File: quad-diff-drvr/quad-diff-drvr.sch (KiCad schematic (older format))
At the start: 53 parts, among them J1 Raspberry_Pi_2_3, J2 Conn_01x04, J3 Conn_01x04, J4 Conn_01x04, J5 Conn_01x04, J6 Conn_01x04, U1 INA3221, U2 74LS153, U3 74LS153, U4 74LS153, U5 PCA9555PW, U6 LTC1688, U7 SLG5NT1581V

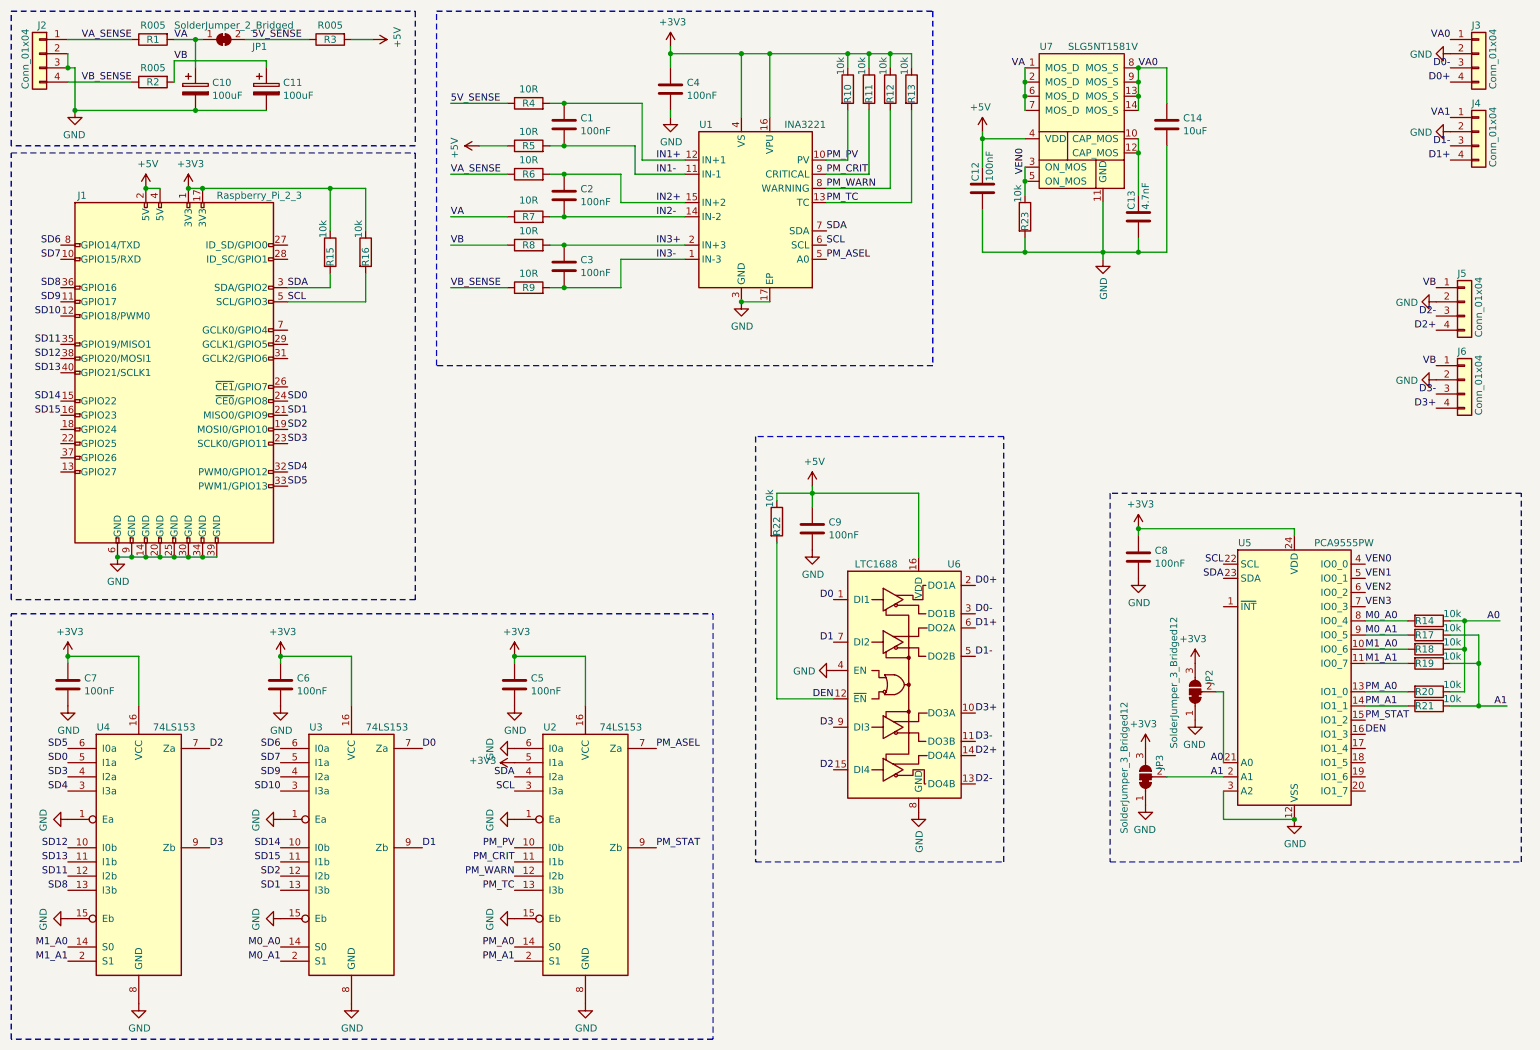
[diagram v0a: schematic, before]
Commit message: qdd: stash wip
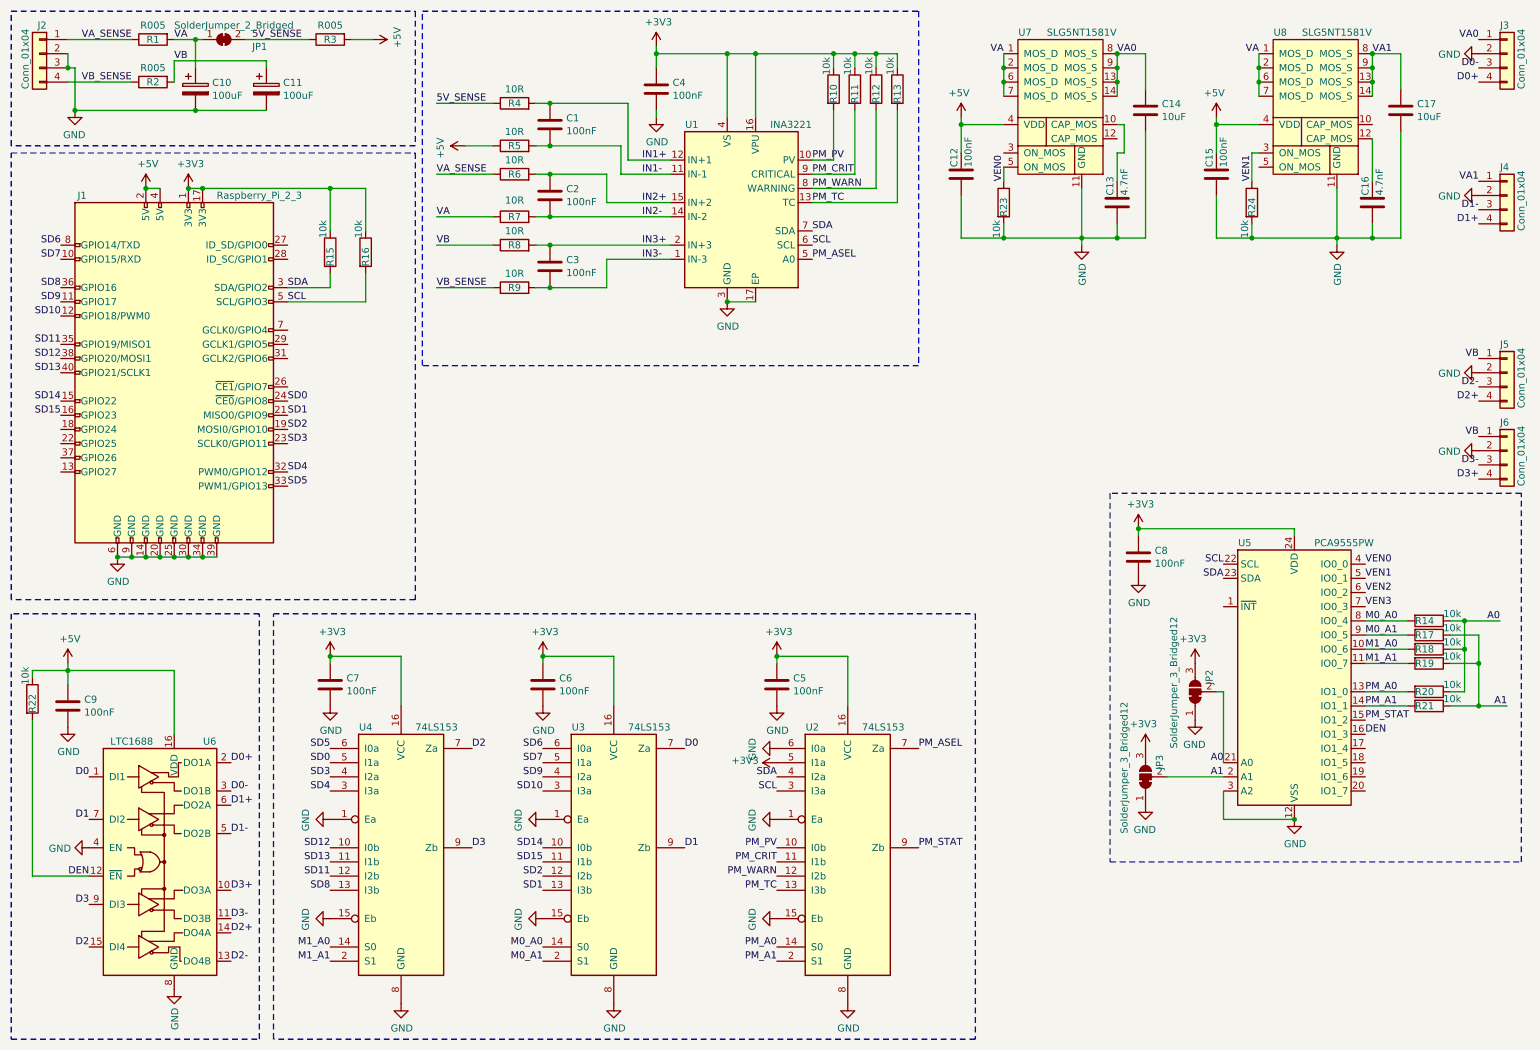
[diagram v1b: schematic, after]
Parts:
- added C15: 100nF, Capacitor_SMD:C_0603_1608Metric, symbol Device:C
- added C16: 4.7nF, Capacitor_SMD:C_0603_1608Metric, symbol Device:C
- added C17: 10uF, Capacitor_SMD:C_0603_1608Metric, symbol Device:C
- added R24: 10k, Resistor_SMD:R_0603_1608Metric, symbol Device:R
- added U8: SLG5NT1581V, octo-pcb:QFN-28_1x3_Pitch0.4mm, symbol octo-pcb:SLG5NT1581V
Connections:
- net +5V: now also C15.1, U8.4 (VDD)
- net GND: now also C15.2, C16.2, C17.2, R24.2, U8.11 (GND)
- net VA: now also U8.1 (MOS_D), U8.2 (MOS_D), U8.6 (MOS_D), U8.7 (MOS_D)
- net VA1: now also C17.1, U8.13 (MOS_S), U8.14 (MOS_S), U8.8 (MOS_S), U8.9 (MOS_S)
- net VEN0: no longer U7.3 (ON_MOS)
- net VEN1: now also R24.1, U8.3 (ON_MOS)
- net at C13.1, U7.10 (CAP_MOS): no longer U7.12 (CAP_MOS)
- new net: C16.1, U8.12 (CAP_MOS)
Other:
- moved on the sheet: C1, C12, C13, C14, C2, C3, C4, C5, C6, C7, C9, J3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
